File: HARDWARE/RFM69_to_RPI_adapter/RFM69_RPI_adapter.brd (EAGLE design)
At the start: 28.9 x 38.1 mm, 3 parts

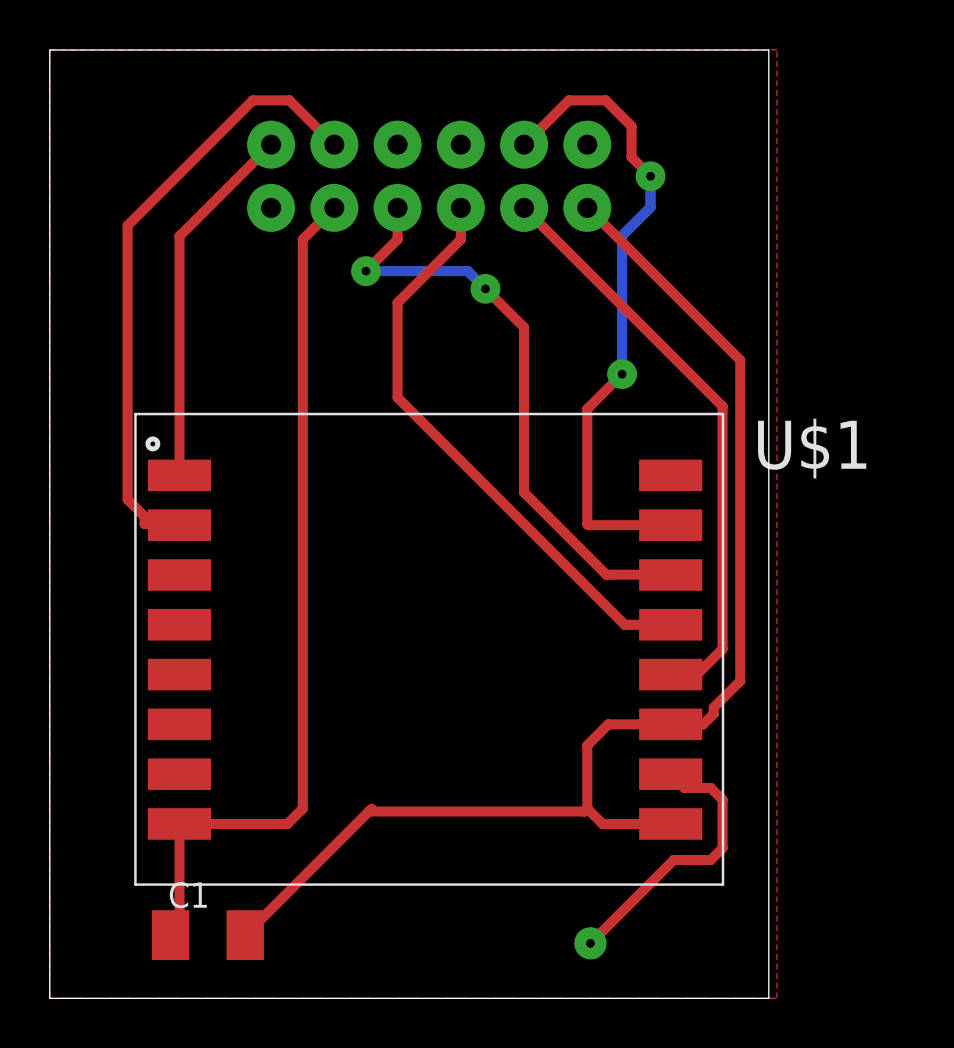
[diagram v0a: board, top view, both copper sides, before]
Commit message: Hardware update
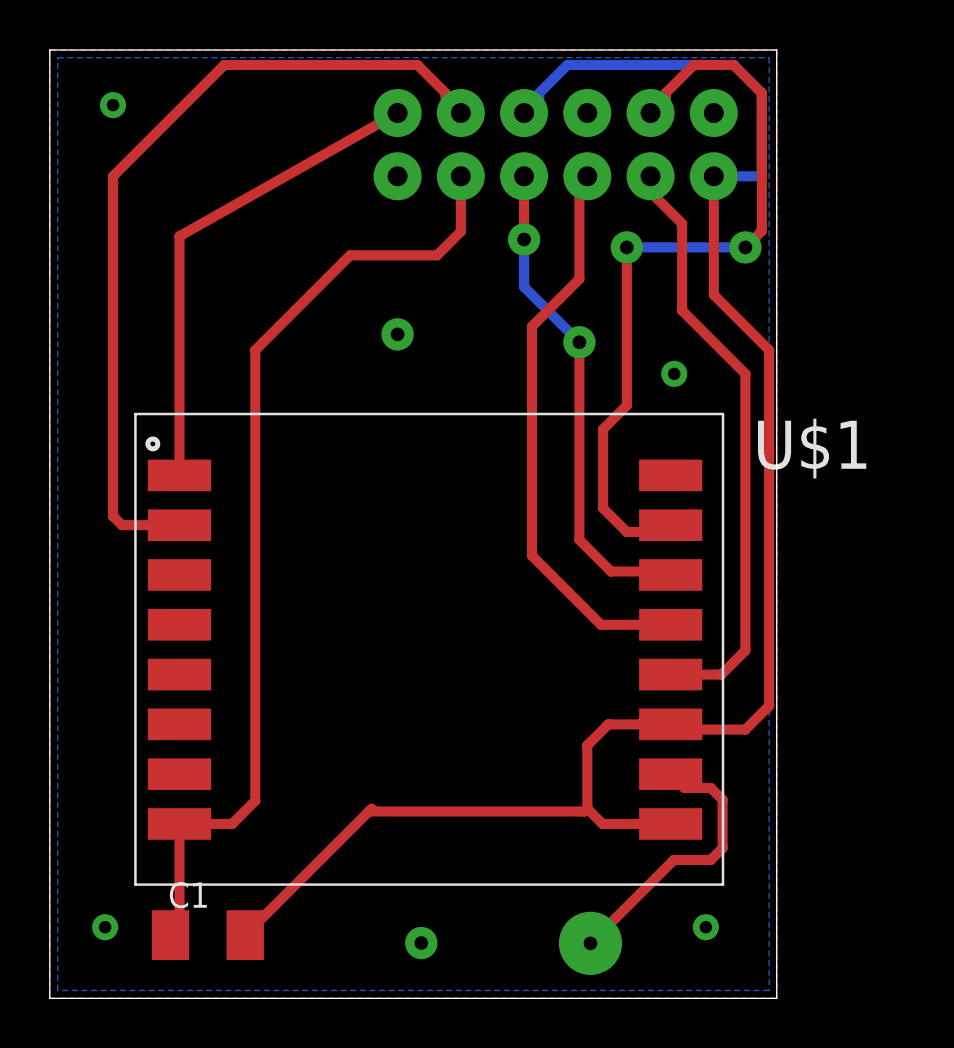
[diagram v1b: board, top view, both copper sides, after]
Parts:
- moved U$2 5.24 mm to (33.0, 57.1)
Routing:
- net GND: track 52.3 -> 69.9 mm, vias 0 -> 2
- net DIO0: track 24.8 -> 33.2 mm
- net CS: track 26.2 -> 31.2 mm
- net RESET: track 14.8 -> 19.7 mm
- net MOSI: track 24.5 -> 20.3 mm
- net VCC: track 34.5 -> 38.6 mm
- net MISO: track 23.4 -> 22.9 mm
- added copper zone on layer 16, net N$7
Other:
- board size 28.9 x 38.1 mm -> 29.2 x 38.1 mm
